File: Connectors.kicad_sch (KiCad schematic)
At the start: 4 parts, among them J1 Conn_01x04_Pin, J2 Conn_01x04_Pin, J3 Conn_01x09_Pin, J4 Conn_02x03_Odd_Even

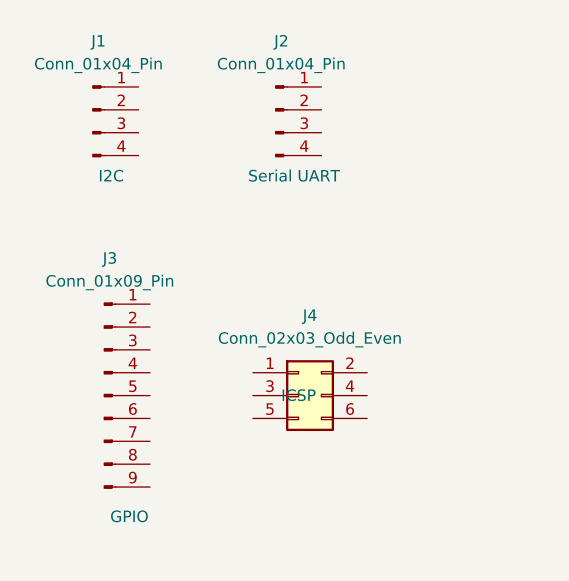
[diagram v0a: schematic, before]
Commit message: Wiring completed
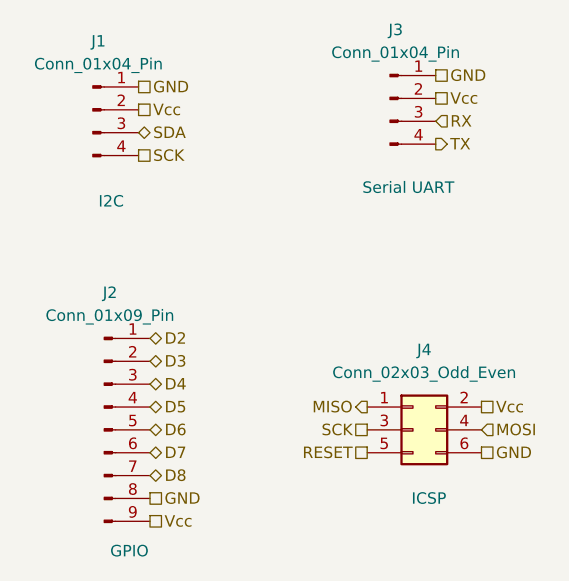
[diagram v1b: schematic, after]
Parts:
- renumbered J3 to J2, J2 to J3
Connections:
- net MISO: now reaches J4.1 (Pin_1)
- net Vcc: now reaches J4.2 (Pin_2)
- net Vcc: now also J1.2 (Pin_2), J2.9 (Pin_9), J3.2 (Pin_2)
- net SCK: now reaches J4.3 (Pin_3)
- net SCK: now also J1.4 (Pin_4)
- net MOSI: now reaches J4.4 (Pin_4)
- net RESET: now reaches J4.5 (Pin_5)
- net GND: now reaches J4.6 (Pin_6)
- net GND: now also J1.1 (Pin_1), J2.8 (Pin_8), J3.1 (Pin_1)
- net SDA: now reaches J1.3 (Pin_3)
- net RX: now reaches J3.3 (Pin_3)
- net TX: now reaches J3.4 (Pin_4)
- net D2: now reaches J2.1 (Pin_1)
- net D3: now reaches J2.2 (Pin_2)
- net D4: now reaches J2.3 (Pin_3)
- net D5: now reaches J2.4 (Pin_4)
- net D6: now reaches J2.5 (Pin_5)
- net D7: now reaches J2.6 (Pin_6)
- net D8: now reaches J2.7 (Pin_7)
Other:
- moved on the sheet: J2, J3, J4
